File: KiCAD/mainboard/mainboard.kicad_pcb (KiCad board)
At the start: 10 copper layers, 130.2 x 81.3 mm, 240 parts, among them IC1 SN74AUP1G06DCKR, IC3 SN74AUP1G06DCKR, IC4 SN74AUP1G07DCKR, IC5 SN74AUP1G07DCKR, J1 AXT550124, J10 Conn_01x05_Pin, J100 AHDF15A-KG-TAXB, J2 Conn_01x07_Pin, J23 B12B-XH-ALFSN, J29 Conn_01x04_Pin, J3 Conn_02x05_Odd_Even, J30 Conn_01x08_Pin, J31 Conn_01x08_Pin, J4 Conn_01x05_Pin, J5 EJ508B, SW2 100SP1T1B4M2QE, U1 XAL5030-472MEC, U12 ECS-2520MV-xxx-xx, U13 MX25L3233FM2, U14 SN74AUP1G06DCKR, U16 DLPC1438ZEZ, U2 LMR33610BDDAR, U22 TXS0102DCU, U24 DLPA2005ERSLT, U26 TPS54340DDA, U3 LMR33610BDDAR, U37 TXS0102DCU, U38 TPD2E001DRYR, U39 TPS62260DDCT, U4 LMR33610BDDAR, U5 SN74AUP1G06DCKR, U6 74AHC1G08, U7 SN74AUP1G06DCKR, U8 74AHC1G32

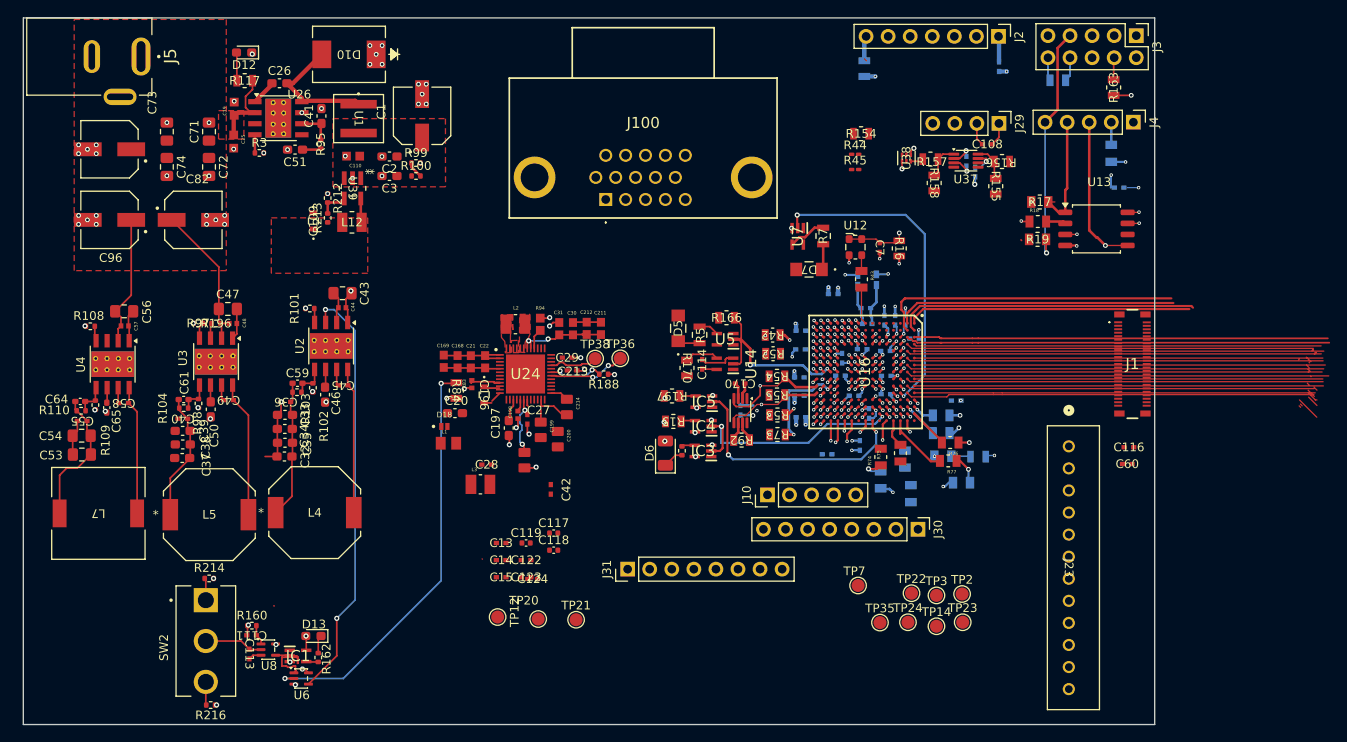
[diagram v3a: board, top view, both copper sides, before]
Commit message: layout
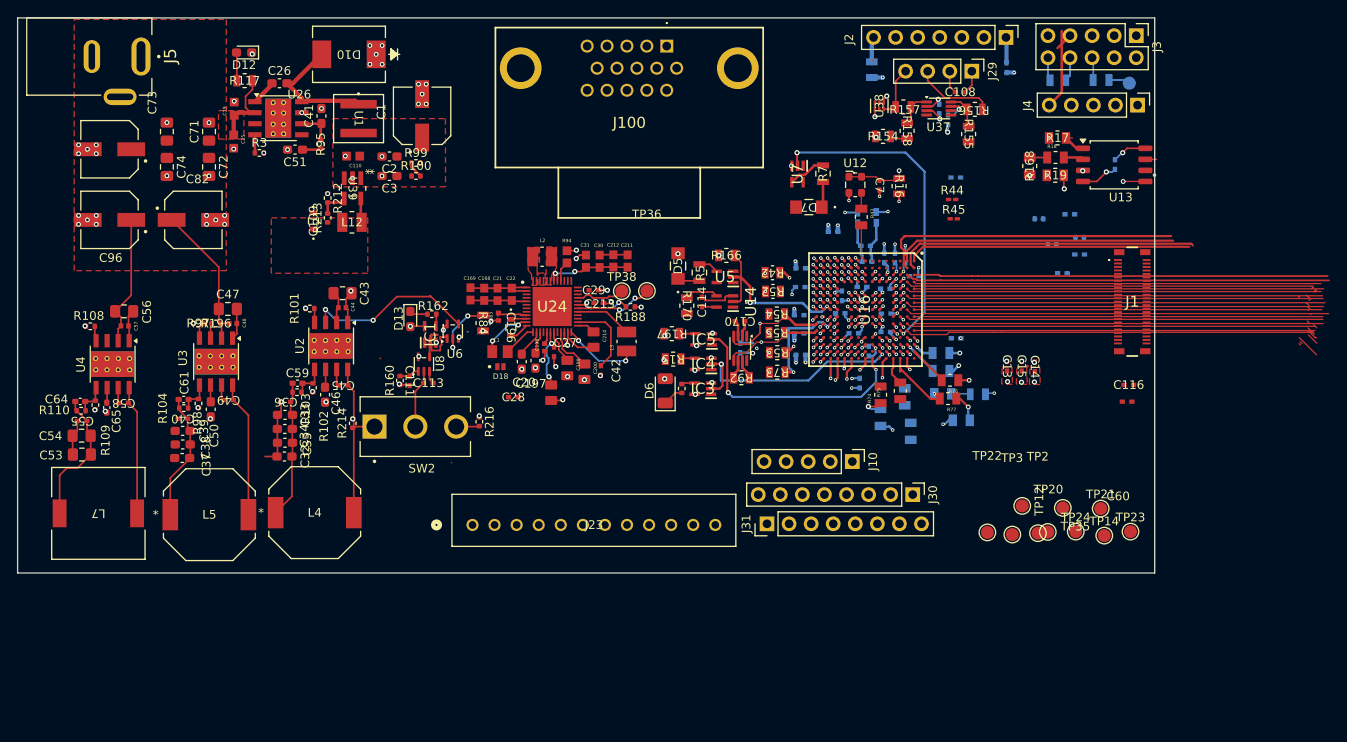
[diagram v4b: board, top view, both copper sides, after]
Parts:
- C117, C118, C119, C122, C123, C124, R163, TP7: moved to B.Cu
- R168: moved to F.Cu
- moved C124 74.7 mm to (210.4, 68.2), turned to 180 degrees
- moved C119 72.8 mm to (211.5, 70.8), turned to 180 degrees
- moved C122 72.8 mm to (211.5, 72.8), turned to 180 degrees
- moved C123 70.9 mm to (209.5, 75.0), turned to 180 degrees
- moved J23 69.2 mm to (141.6, 103.9), turned to 0 degrees
- moved C118 67.3 mm to (208.3, 71.7), turned to 180 degrees
- moved C117 66.5 mm to (206.8, 68.7), turned to 180 degrees
- moved TP7 65.7 mm to (217.2, 53.1), turned to 180 degrees
- moved C14 65.3 mm to (206.3, 85.7), turned to -90 degrees
- moved C15 64.6 mm to (204.8, 85.7), turned to -90 degrees
- moved TP12 61.7 mm to (204.9, 101.7)
- moved TP20 61.7 mm to (209.6, 102.0)
- moved TP21 61.7 mm to (213.9, 102.0)
- moved C13 61.7 mm to (203.2, 85.7), turned to -90 degrees
- moved R216 44.9 mm to (142.4, 92.0), turned to -90 degrees
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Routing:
- net /DLPC1438_Interface/INTZ: track 48.7 -> 7.71 mm
- net /Power_Input&Generation/FPGA_PWREN: track 48.8 -> 19.9 mm
- net /DLPC1438_Interface/SPI0_MOSI: track 21.7 -> 6.70 mm
- net /DLPC1438_Interface/SPI0_CLK: track 29.1 -> 14.2 mm
- net /DLPC1438_Interface/SPI0_CSZ0: track 15.2 -> 4.77 mm
- net /DLPC1438_Interface/EXT_SCL: track 0.00 -> 9.27 mm
- net /DLPA2005_Interface/PWM_IN: track 0.00 -> 8.90 mm
- net /DLPA2005_Interface/SWC: track 0.00 -> 8.89 mm, vias 0 -> 2
- net P1P1V: track 22.7 -> 29.4 mm
- net /DLPA2005_Interface/SWN: track 0.00 -> 6.28 mm, vias 0 -> 2
- net Net-(U24-LS_OUT): track 0.00 -> 5.26 mm
- net /DLPC1438_Interface/EXT_SDA: track 1.49 -> 6.07 mm
- net /DLPA2005_Interface/<NO NET>: track 0.00 -> 3.85 mm
- net /DLPA2005_Interface/VRST: track 0.06 -> 3.23 mm
- net GND: track 142.6 -> 140.3 mm, vias 162 -> 168
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- added copper zone on F.Cu, net /DLPA2005_Interface/VRST
- added copper zone on F.Cu, net VBIAS
- added copper zone on F.Cu, net VOFS
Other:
- board size 130.2 x 81.3 mm -> 130.9 x 63.9 mm
